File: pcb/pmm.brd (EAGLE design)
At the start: 30 x 35 mm, 12 parts, among them IC2 REG1117, IC3 STM32F042F4, U2 USBC_16P

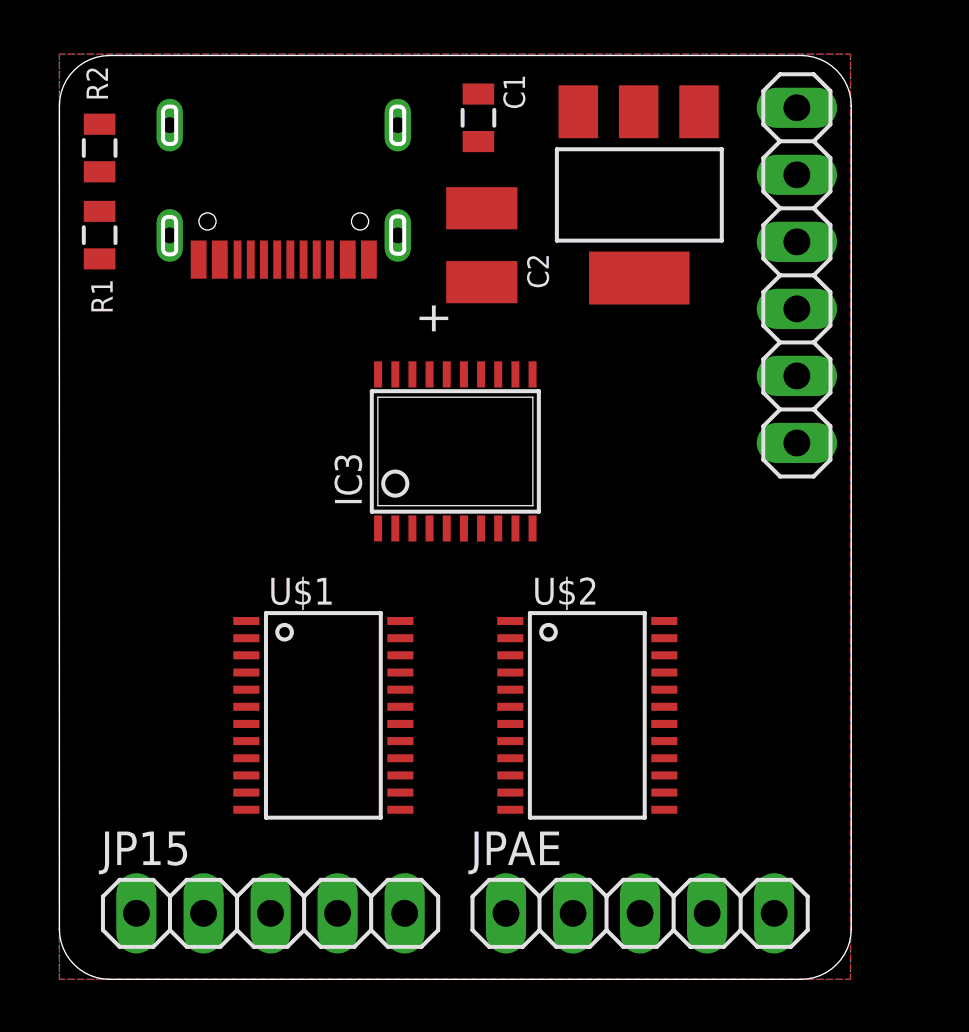
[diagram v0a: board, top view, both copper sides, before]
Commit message: pcb done
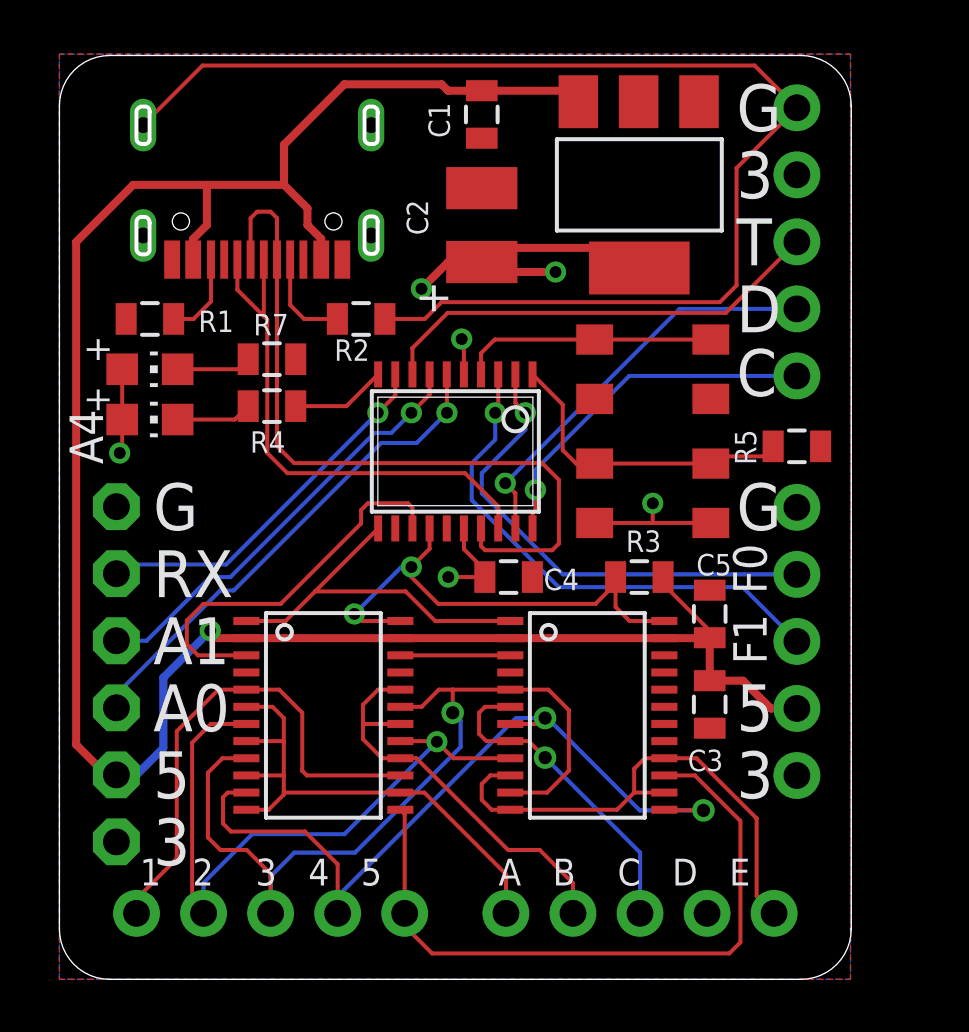
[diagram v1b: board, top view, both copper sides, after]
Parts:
- removed JP15, JPAE: (no value), pinhead:1X05
- added C3, C5: 10uF, clock:0805@1
- added C4: 100nF, clock:0805@1
- added LED1, LED2: (no value), adafruit:CHIP-LED0805
- added R3, R5: 10K, joyAnalog:0805
- added R4, R7: 2K, SparkFun-Passives:0805
- added SW3, SW4: 324_SW, 3pos_slide_switch_centered:342_SWICH_FOOT
- added U$3, U$4, U$5, U$6: PINHD5, adafruit_changed:1X05
- C1: value 100nF -> 10uF
- JP1: device pinhead:1X06 -> adafruit:1X06-CLEANBIG
- moved JP1 29.9 mm to (2.16, 11.6), turned to 270 degrees
- moved R2 11.8 mm to (11.4, 25.0), turned to 0 degrees
- moved R1 3.70 mm to (3.43, 25.0), turned to 180 degrees
- moved U2 1.01 mm to (7.49, 31.1)
- moved C2 0.76 mm to (16.0, 28.6)
- moved IC2 0.38 mm to (22.0, 30.1)
- moved C1 0.18 mm to (16.0, 32.8), turned to 90 degrees
- turned IC3 to 180 degrees
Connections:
- removed net DNDNDN: U2.A7, U2.B7
- new net +5V: C1.2, C3.2, C5.2, IC2.3, JP1.5, R3.2, U$1.2, U$1.23, U$2.2, U$2.23, U$5.4, U2.A4B9, U2.B4A9
- new net BUTTON1: IC3.4, SW3.P$2, SW3.P$3
- new net BUTTON2: IC3.1, R5.2, SW4.P$2, SW4.P$3
- new net N$10: IC3.7, JP1.3
- new net N$11: IC3.6, JP1.4
- new net N$12: IC3.2, U$5.2
- new net N$13: IC3.3, U$5.3
- new net N$2: IC3.13, U$1.3
- new net N$29: LED2.C, R7.2
- new net N$3: U$1.22, U$2.3
- new net N$4: IC3.14, R3.1, U$1.24, U$2.24
- new net N$5: LED1.C, R4.2
- new net N$6: IC3.8, U$6.3
- new net N$7: IC3.20, U$6.1
- new net N$8: IC3.19, U$6.2
- new net N$9: IC3.9, JP1.2
- new net USB_DN: IC3.17, U2.A7, U2.B7
- new net USER_LED: IC3.10, R4.1
- net +3V3: now also C4.2, IC3.16, IC3.5, JP1.6, LED1.A, LED2.A, SW4.P$1, SW4.P$4, U$5.5, U$6.4; no longer JP1.4
- net 1: now also U$3.1; no longer JP15.1
- net 2: now also U$3.2; no longer JP15.2
- net 3: now also U$3.3; no longer JP15.3
- net 4: now also U$3.4; no longer JP15.4
- net 5: now also U$3.5; no longer JP15.5
- net A: now also U$4.1; no longer JPAE.1
- net B: now also U$4.2; no longer JPAE.2
- net C: now also U$4.3; no longer JPAE.3
- net E: now also U$4.5; no longer JPAE.5
- net GND: now also C3.1, C4.1, C5.1, IC3.15, JP1.1, R5.1, R7.1, SW3.P$1, SW3.P$4, U$1.21, U$1.4, U$2.21, U$2.4, U$5.1, U$6.5; no longer JP1.5
- net N$1: now also IC3.11, U$1.1, U$2.1; no longer C1.2, IC2.3, U2.A4B9, U2.B4A9
- net USB_DP: now also IC3.18
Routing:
- net +5V: track 0.00 -> 85.0 mm, vias 0 -> 1
- net GND: track 0.00 -> 47.9 mm
- net 3: track 0.00 -> 33.3 mm, vias 0 -> 1
- net 4: track 0.00 -> 30.4 mm, vias 0 -> 2
- net USB_DN: track 0.00 -> 28.8 mm
- net 5: track 0.00 -> 26.0 mm
- net 2: track 0.00 -> 25.6 mm, vias 0 -> 1
- net +3V3: track 0.00 -> 25.5 mm, vias 0 -> 6
- net USB_DP: track 0.00 -> 20.4 mm
- net A: track 0.00 -> 20.2 mm
- net N$13: track 0.00 -> 19.7 mm, vias 0 -> 1
- net E: track 0.00 -> 19.7 mm
- net 1: track 0.00 -> 19.3 mm
- net N$11: track 0.00 -> 18.9 mm, vias 0 -> 1
- net N$4: track 0.00 -> 18.8 mm, vias 0 -> 2
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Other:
- board text added: "1 2 3 4 5"
- board text added: "3"
- board text added: "5"
- board text added: "A B C D E"
- board text added: "A0"
- board text added: "A1"
- board text added: "A4"
- board text added: "C"
- board text added: "D"
- board text added: "F0"
- board text added: "F1"
- board text added: "G"
- board text added: "Pimp-my-microwave dekuNukem JUL2020 PT0"
- board text added: "RX"
- board text added: "T"
